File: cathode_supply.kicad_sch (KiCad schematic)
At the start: 15 parts, among them Q4 IRF540SPBF, U8 INA180A3

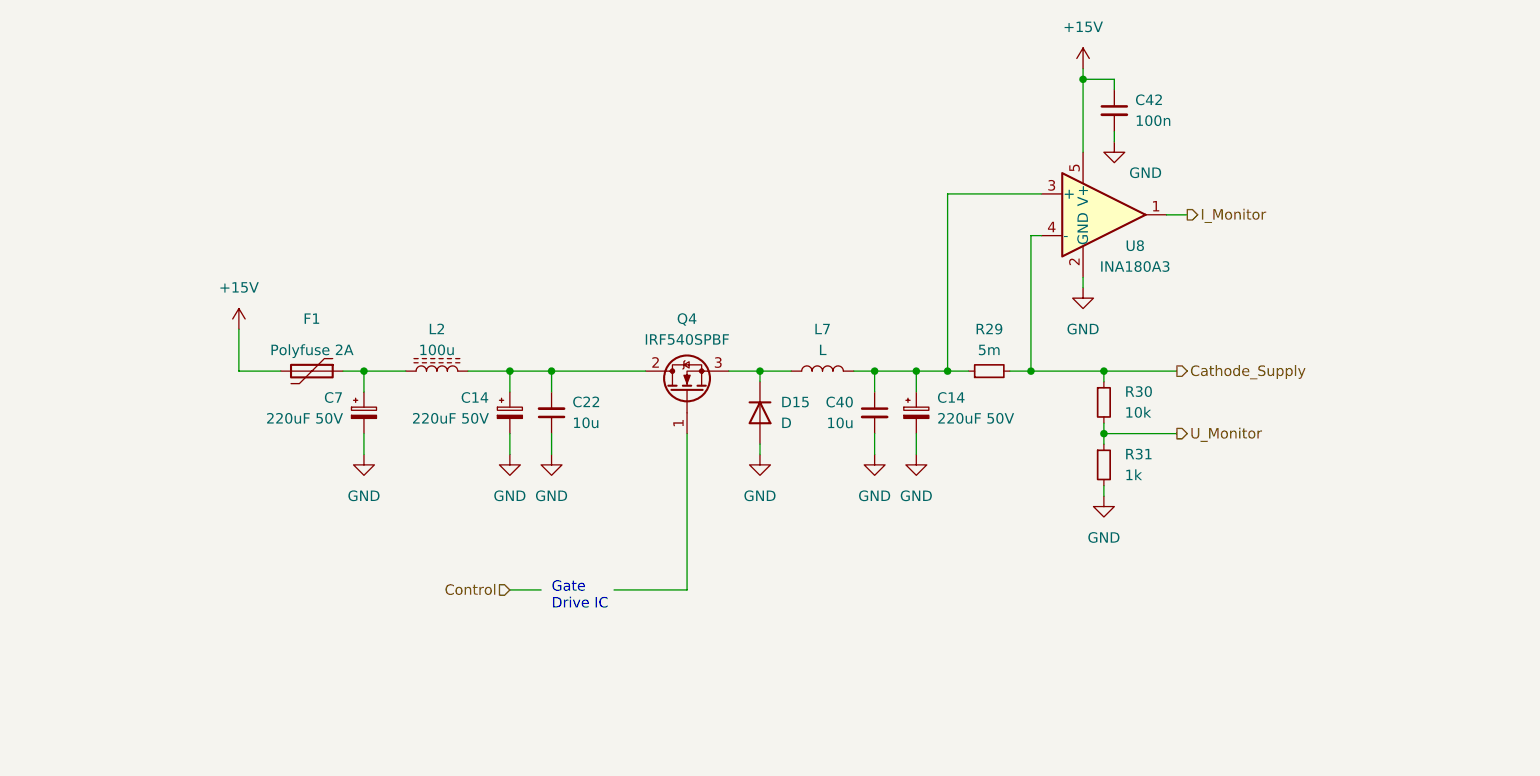
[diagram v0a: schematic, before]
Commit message: A lot of work
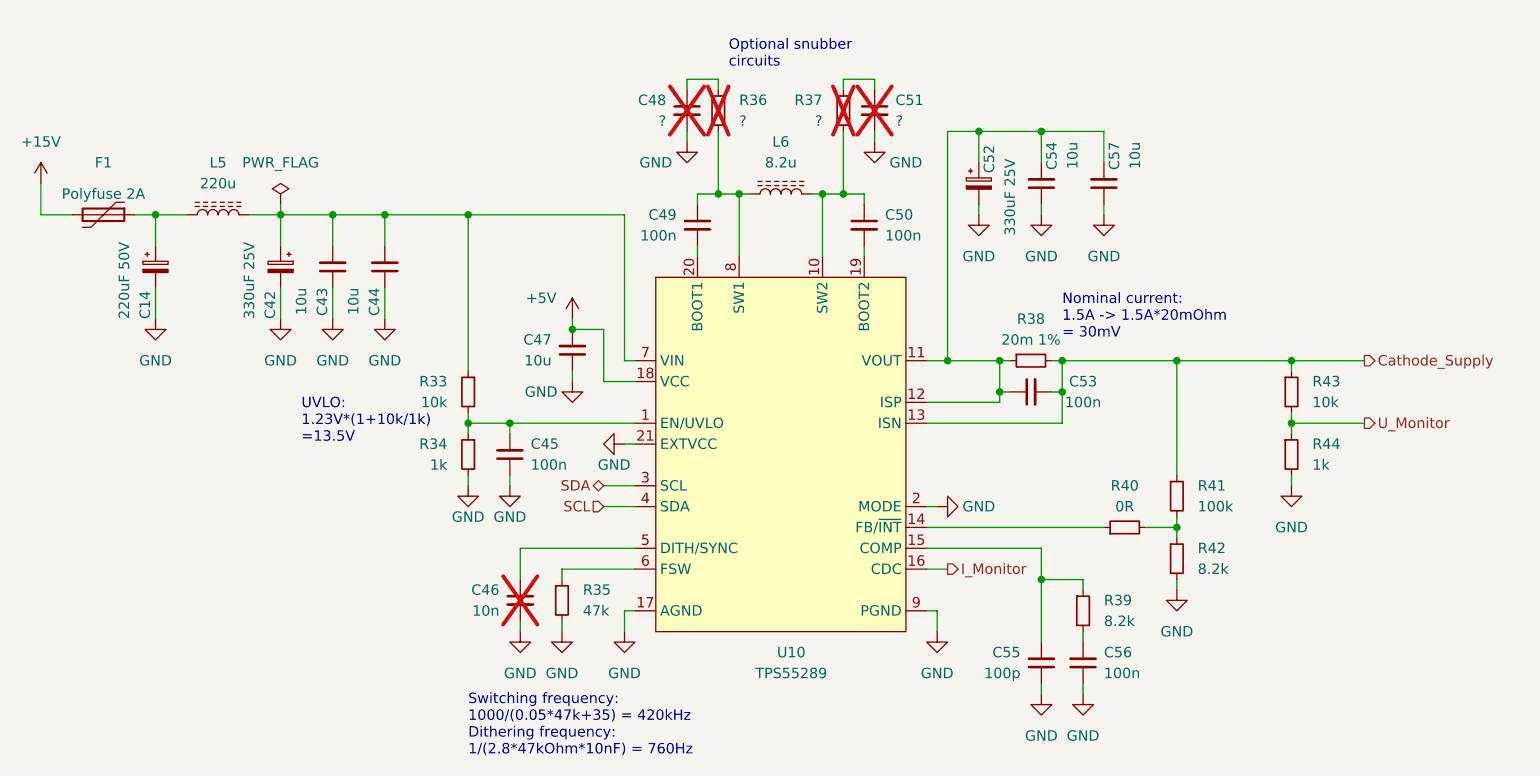
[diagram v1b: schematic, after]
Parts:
- removed C14 (x2), C7: 220uF 50V, Capacitor_SMD:CP_Elec_6.3x7.7, symbol MEMS_Passive:C_Elec-220uf-50V
- removed C22, C40: 10u, symbol Device:C_Small
- removed C42: 100n, symbol Device:C_Small
- removed D15: D, symbol Device:D
- removed L2: 100u, MEMS_Passive:L_Bourns_PM2110, symbol MEMS_Passive:L_100u_choke
- removed L7: L, symbol Device:L
- removed Q4: IRF540SPBF, Package_TO_SOT_SMD:TO-263-2, symbol MEMS_Discrete-semiconductor:Q_IRF540SP
- removed R29: 5m, symbol Device:R_Small
- removed U8: INA180A3, Package_TO_SOT_SMD:SOT-23-5, symbol Amplifier_Current:INA180A3
- added C14: 220uF 50V, Capacitor_SMD:CP_Elec_6.3x7.7, symbol MEMS_Passive:C_Elec-220uf-50V
- added C42, C52: 330uF 25V, Capacitor_SMD:CP_Elec_10x12.5, symbol MEMS_Passive:C_Elec-330uF-25V
- added C43, C44, C47, C54, C57: 10u, Capacitor_SMD:C_0805_2012Metric_Pad1.18x1.45mm_HandSolder, symbol Device:C_Small
- added C45, C49, C50, C53, C56: 100n, Capacitor_SMD:C_0805_2012Metric_Pad1.18x1.45mm_HandSolder, symbol Device:C_Small
- added C46: 10n, Capacitor_SMD:C_0805_2012Metric_Pad1.18x1.45mm_HandSolder, symbol Device:C_Small
- added C48, C51: ?, Capacitor_SMD:C_0805_2012Metric_Pad1.18x1.45mm_HandSolder, symbol Device:C_Small
- added C55: 100p, Capacitor_SMD:C_0805_2012Metric_Pad1.18x1.45mm_HandSolder, symbol Device:C_Small
- added L5: 220u, Inductor_SMD:L_12x12mm_H8mm, symbol MEMS_Passive:L_220u_10x10
- added L6: 8.2u, MEMS_Passive:L_Bourns_SRP7030, symbol MEMS_Passive:L_8.2u_5.9/10.2A
- added R33: 10k, Resistor_SMD:R_0805_2012Metric_Pad1.20x1.40mm_HandSolder, symbol Device:R_Small
- added R34: 1k, Resistor_SMD:R_0805_2012Metric_Pad1.20x1.40mm_HandSolder, symbol Device:R_Small
- added R35: 47k, Resistor_SMD:R_0805_2012Metric_Pad1.20x1.40mm_HandSolder, symbol Device:R_Small
- added R36, R37: ?, Resistor_SMD:R_0805_2012Metric_Pad1.20x1.40mm_HandSolder, symbol Device:R_Small
- added R38: 20m 1%, Resistor_SMD:R_2010_5025Metric_Pad1.40x2.65mm_HandSolder, symbol MEMS_Passive:R_2010_20m_1%
- added R39, R42: 8.2k, Resistor_SMD:R_0805_2012Metric_Pad1.20x1.40mm_HandSolder, symbol Device:R_Small
- added R40: 0R, Resistor_SMD:R_0805_2012Metric_Pad1.20x1.40mm_HandSolder, symbol Device:R_Small
- added R41: 100k, Resistor_SMD:R_0805_2012Metric_Pad1.20x1.40mm_HandSolder, symbol Device:R_Small
- added U10: TPS55289, MEMS_IC:TPS55289, symbol MEMS_IC:TPS55289
- R43: renamed from R30; footprint (none) -> Resistor_SMD:R_0805_2012Metric_Pad1.20x1.40mm_HandSolder
- R44: renamed from R31; footprint (none) -> Resistor_SMD:R_0805_2012Metric_Pad1.20x1.40mm_HandSolder
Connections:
- net Cathode_Supply: now also C53.2, R38.2, R41.1, U10.13 (ISN)
- net GND: now also C14.2, C42.2, C43.1, C44.1, C45.1, C46.2, C47.1, C48.2, C51.2, C52.2, C54.1, C55.1, C56.1, C57.1, R34.2, R35.2, R42.2, U10.17 (AGND), U10.2 (MODE), U10.21 (EXTVCC), U10.9 (PGND)
- net I_Monitor: now also U10.16 (CDC)
- net at F1.1: now also C14.1, L5.1
- new net: C52.1, C53.1, C54.2, C57.2, R38.1, U10.11 (VOUT), U10.12 (ISP)
- new net: C48.1, R36.1
- new net: C51.1, R37.1
- new net: C42.1, C43.2, C44.2, L5.2, R33.1, U10.7 (VIN)
- new net: R35.1, U10.6 (FSW)
- new net: C50.1, L6.2, R37.2, U10.10 (SW2)
- new net: R40.2, R41.2, R42.1
- new net: R40.1, U10.14 (FB/~{INT})
- new net: C49.1, L6.1, R36.2, U10.8 (SW1)
- new net: C49.2, U10.20 (BOOT1)
- new net: C45.2, R33.2, R34.1, U10.1 (EN/UVLO)
- new net: C55.2, R39.1, U10.15 (COMP)
- new net: C50.2, U10.19 (BOOT2)
- new net: C46.1, U10.5 (DITH/SYNC)
- new net: C56.2, R39.2
- new net +5V: C47.2, U10.18 (VCC)
- new net SCL: U10.4 (SDA)
- new net SDA: U10.3 (SCL)
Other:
- note added: "Nominal current: 1.5A -> 1.5A*20mOhm = 30mV"
- note added: "Optional snubber circuits"
- note added: "Switching frequency: 1000/(0.05*47k+35) = 420kHz Dithering frequency: 1/(2.8*47kOhm*10nF) = 760Hz"
- note added: "UVLO: 1.23V*(1+10k/1k) =13.5V"
- note removed: "Gate Drive IC"
- title: (none) -> EuroMeasure Ion Gauge Controller
- moved on the sheet: R43, R44
